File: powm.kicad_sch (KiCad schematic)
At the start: 35 parts, among them J1 USB_C_Receptacle_PowerOnly_6P, Q1 IRLR2905, Q2 IRLR2905, Q3 IRLR2905, Q4 IRLR2905, Q5 IRLR2905, U1 IP2721, U3 BQ25792

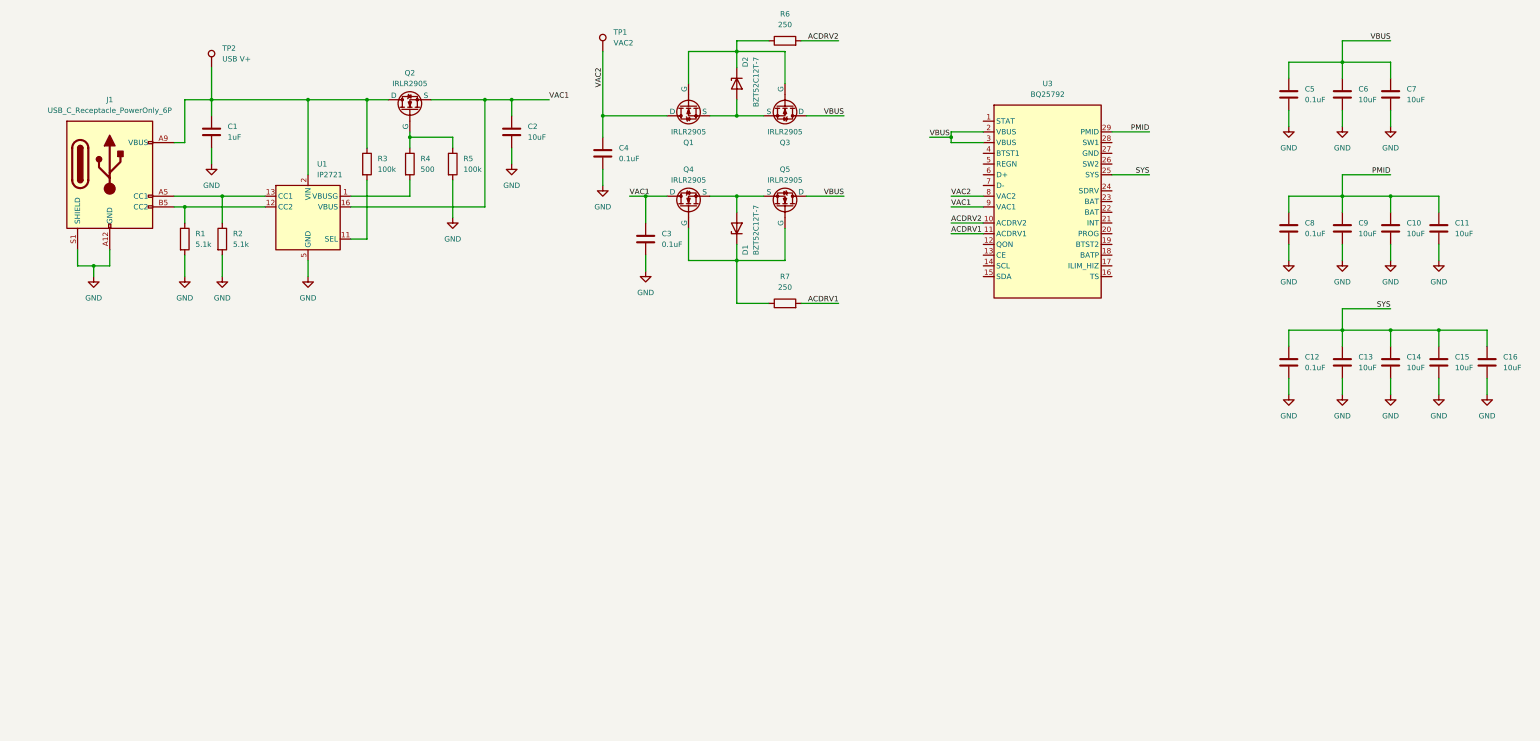
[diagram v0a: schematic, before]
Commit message: 4
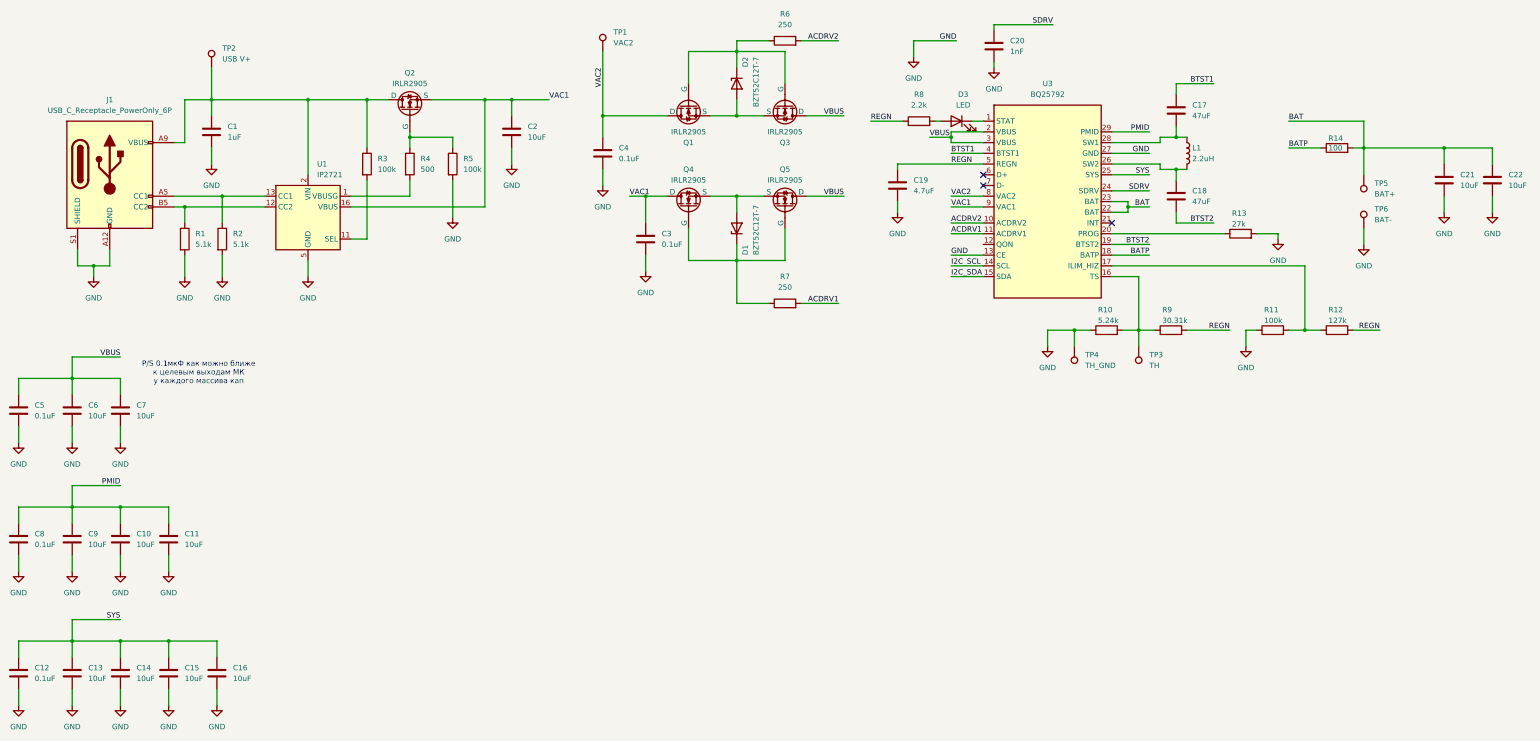
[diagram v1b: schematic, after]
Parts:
- added C17, C18: 47uF, Capacitor_SMD:C_0603_1608Metric_Pad1.08x0.95mm_HandSolder, symbol Device:C
- added C19: 4.7uF, Capacitor_SMD:C_0603_1608Metric_Pad1.08x0.95mm_HandSolder, symbol Device:C
- added C20: 1nF, Capacitor_SMD:C_0603_1608Metric_Pad1.08x0.95mm_HandSolder, symbol Device:C
- added C21, C22: 10uF, Capacitor_SMD:C_0603_1608Metric_Pad1.08x0.95mm_HandSolder, symbol Device:C
- added D3: LED, symbol Device:LED
- added L1: 2.2uH, symbol Device:L
- added R10: 5.24k, Resistor_SMD:R_0603_1608Metric_Pad0.98x0.95mm_HandSolder, symbol Device:R
- added R11: 100k, Resistor_SMD:R_0603_1608Metric_Pad0.98x0.95mm_HandSolder, symbol Device:R
- added R12: 127k, Resistor_SMD:R_0603_1608Metric_Pad0.98x0.95mm_HandSolder, symbol Device:R
- added R13: 27k, Resistor_SMD:R_0603_1608Metric_Pad0.98x0.95mm_HandSolder, symbol Device:R
- added R14: 100, Resistor_SMD:R_0603_1608Metric_Pad0.98x0.95mm_HandSolder, symbol Device:R
- added R8: 2.2k, Resistor_SMD:R_0603_1608Metric_Pad0.98x0.95mm_HandSolder, symbol Device:R
- added R9: 30.31k, Resistor_SMD:R_0603_1608Metric_Pad0.98x0.95mm_HandSolder, symbol Device:R
- added TP3: TH, TestPoint:TestPoint_THTPad_D2.0mm_Drill1.0mm, symbol Connector:TestPoint
- added TP4: TH_GND, TestPoint:TestPoint_THTPad_D2.0mm_Drill1.0mm, symbol Connector:TestPoint
- added TP5: BAT+, TestPoint:TestPoint_THTPad_D2.0mm_Drill1.0mm, symbol Connector:TestPoint
- added TP6: BAT-, TestPoint:TestPoint_THTPad_D2.0mm_Drill1.0mm, symbol Connector:TestPoint
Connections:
- net GND: now also U3.13 (CE), U3.27 (GND), C19.2, C20.2, C21.2, C22.2, R10.1, R11.1, R13.2, TP4.1, TP6.1
- net at U3.1 (STAT): now also D3.1 (K)
- net I2C_SCL: now reaches U3.14 (SCL)
- net I2C_SDA: now reaches U3.15 (SDA)
- net at U3.16 (TS): now also R10.2, R9.1, TP3.1
- net at U3.17 (ILIM_HIZ): now also R11.2, R12.1
- net BATP: now reaches U3.18 (BATP)
- net BATP: now also R14.1
- net BTST2: now reaches U3.19 (BTST2)
- net BTST2: now also C18.2
- net at U3.20 (PROG): now also R13.1
- net BAT: now reaches U3.22 (BAT)
- net BAT: now also U3.23 (BAT), C21.1, C22.1, R14.2, TP5.1
- net SDRV: now reaches U3.24 (SDRV)
- net SDRV: now also C20.1
- net at U3.26 (SW2): now also C18.1, L1.2
- net at U3.28 (SW1): now also C17.2, L1.1
- net BTST1: now reaches U3.4 (BTST1)
- net BTST1: now also C17.1
- net REGN: now reaches U3.5 (REGN)
- net REGN: now also C19.1, R12.2, R8.1, R9.2
- new net: D3.2 (A), R8.2
- no-connect marks 0 -> 3
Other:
- note added: "P/S 0.1мкФ как можно ближе к целевым выходам МК у каждого массива кап"
- moved on the sheet: C10, C11, C12, C13, C14, C15, C16, C5, C6, C7, C8, C9
